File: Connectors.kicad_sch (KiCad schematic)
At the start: 23 parts, among them J1 Precidip 853-87-004-20-001101, J10 Precidip 853-87-004-20-001101, J11 7 pin FPC 0.3mm Aces 51688-00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, J12 Precidip 853-87-004-20-001101, J13 TE 3-2363961-0 receptacle, J15 Precidip 853-87-004-20-001101, J16 TE 3-2363961-0 receptacle, J18 Precidip 852-10-004-20-001101, J2 Precidip 853-87-004-20-001101, J3 7 pin FPC 0.3mm Aces 51688-00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, J4 Precidip 853-87-004-20-001101, J5 7 pin FPC 0.3mm Aces 51688-00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, J6 Precidip 853-87-004-20-001101, J7 Precidip 853-87-004-20-001101, J8 7 pin FPC 0.3mm Aces 51688-00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, J9 Precidip 853-87-004-20-001101

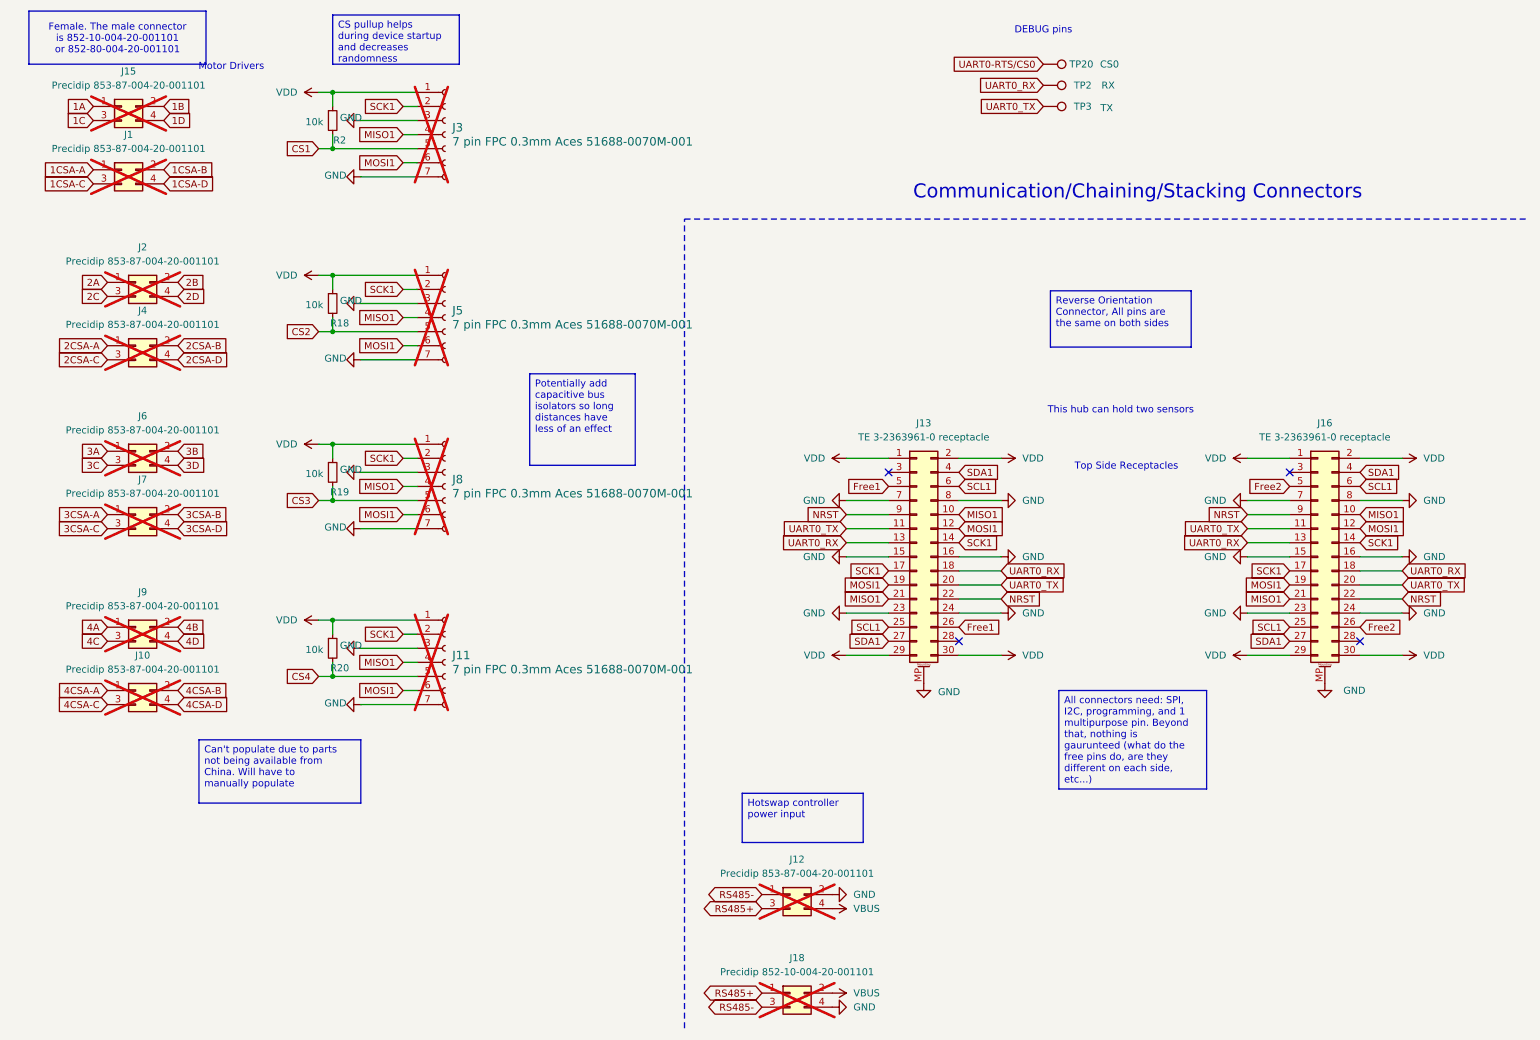
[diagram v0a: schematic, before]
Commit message: Improve schematic consistency
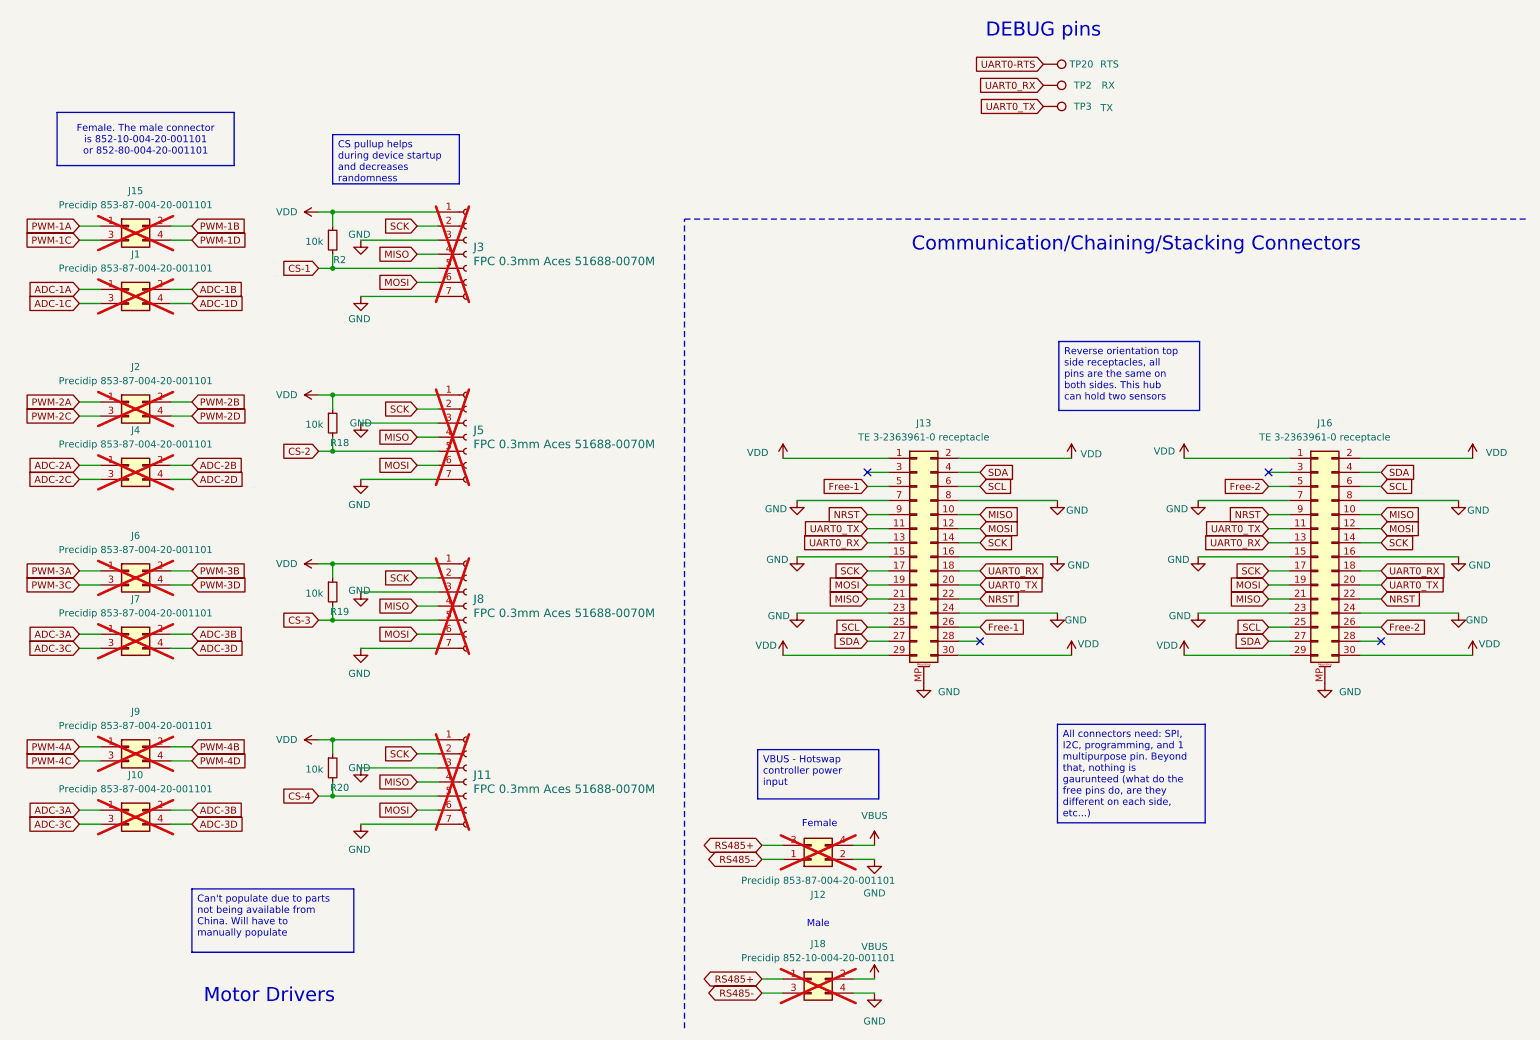
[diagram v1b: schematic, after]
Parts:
- J11, J3, J5, J8: value 7 pin FPC 0.3mm Aces 51688-0070M-001 -> FPC 0.3mm Aces 51688-0070M
- TP20: value CS0 -> RTS
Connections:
- net 4CSA-A is gone; now on net ADC-3A: J10.1 (Pin_1)
- net 4CSA-B is gone; now on net ADC-3B: J10.2 (Pin_2)
- net 4CSA-C is gone; now on net ADC-3C: J10.3 (Pin_3)
- net 4CSA-D is gone; now on net ADC-3D: J10.4 (Pin_4)
- net 1A renamed PWM-1A
- net 1B renamed PWM-1B
- net 1C renamed PWM-1C
- net 1CSA-A renamed ADC-1A
- net 1CSA-B renamed ADC-1B
- net 1CSA-C renamed ADC-1C
- net 1CSA-D renamed ADC-1D
- net 1D renamed PWM-1D
- net 2A renamed PWM-2A
- net 2B renamed PWM-2B
- net 2C renamed PWM-2C
- net 2CSA-A renamed ADC-2A
- net 2CSA-B renamed ADC-2B
- net 2CSA-C renamed ADC-2C
- net 2CSA-D renamed ADC-2D
- net 2D renamed PWM-2D
- net 3A renamed PWM-3A
- net 3B renamed PWM-3B
- net 3C renamed PWM-3C
- net 3CSA-A renamed ADC-3A
- net 3CSA-B renamed ADC-3B
- net 3CSA-C renamed ADC-3C
- net 3CSA-D renamed ADC-3D
- net 3D renamed PWM-3D
- net 4A renamed PWM-4A
- net 4B renamed PWM-4B
- net 4C renamed PWM-4C
- net 4D renamed PWM-4D
- net CS1 renamed CS-1
- net CS2 renamed CS-2
- net CS3 renamed CS-3
- net CS4 renamed CS-4
- net Free1 renamed Free-1
- net Free2 renamed Free-2
- net MISO1 renamed MISO
- net MOSI1 renamed MOSI
- net SCK1 renamed SCK
- net SCL1 renamed SCL
- net SDA1 renamed SDA
- net UART0-RTS/CS0 renamed UART0-RTS
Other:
- note added: "Female"
- note added: "Male"
- note removed: "This hub can hold two sensors"
- note removed: "Top Side Receptacles"
- moved on the sheet: J1, J10, J11, J12, J15, J18, J2, J3, J4, J5, J6, J7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
